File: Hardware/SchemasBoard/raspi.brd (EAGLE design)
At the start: 14.2 x 24.8 mm, 9 parts

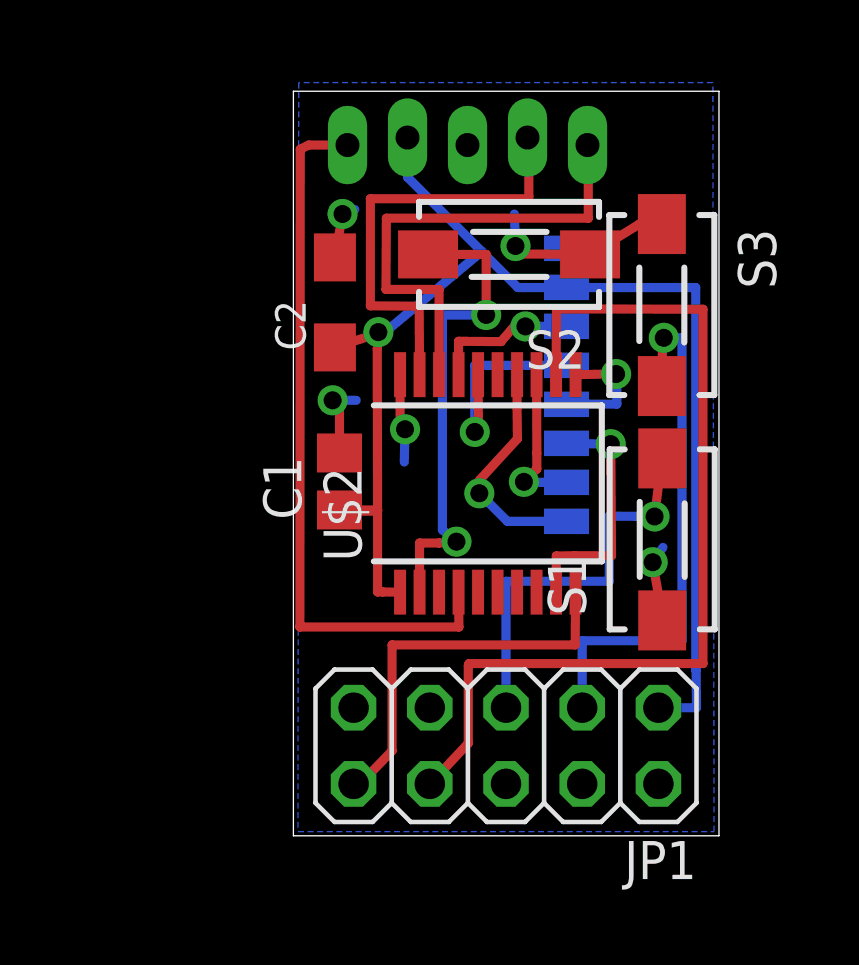
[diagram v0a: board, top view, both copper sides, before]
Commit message: aaa
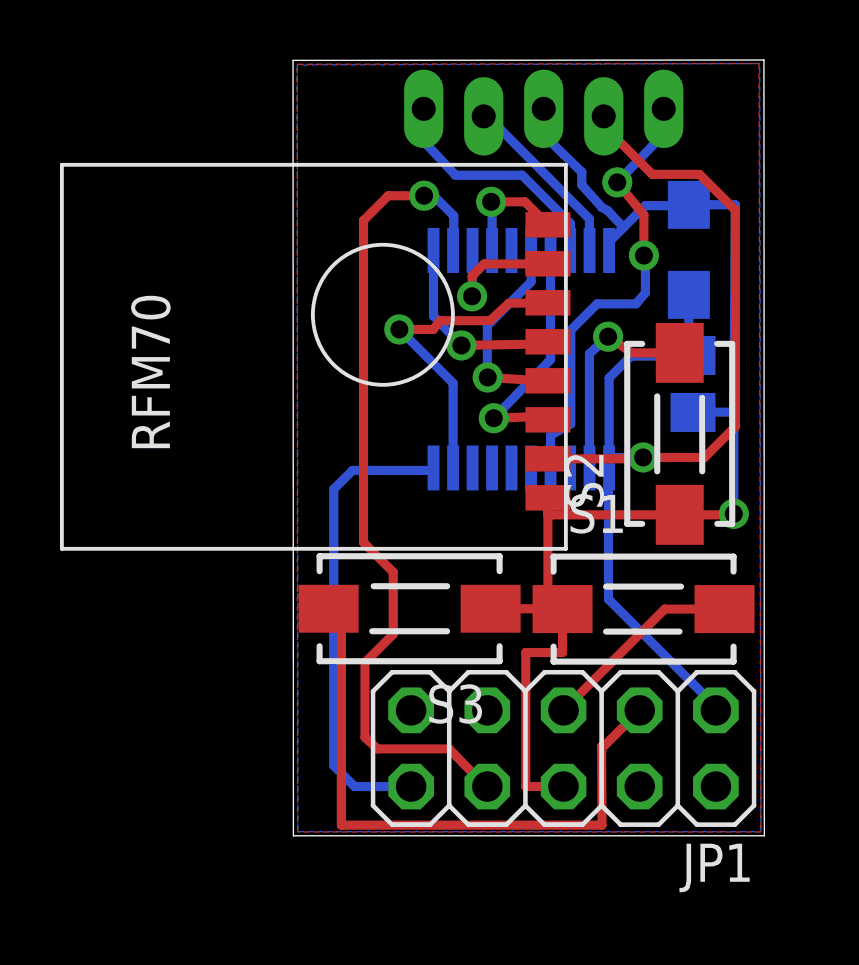
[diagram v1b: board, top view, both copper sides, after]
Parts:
- moved S3 13.2 mm to (3.87, 7.57), turned to 180 degrees
- moved C1 12.2 mm to (13.3, 15.1), flipped to the bottom, turned to 270 degrees
- moved C2 11.9 mm to (13.2, 19.5), flipped to the bottom
- moved S2 8.26 mm to (12.9, 13.4), turned to 90 degrees
- moved U$1 8.14 mm to (-5.82, 11.4), flipped to the top, turned to 90 degrees
- moved U$2 4.29 mm to (7.60, 15.9), flipped to the bottom
- moved U$3 2.81 mm to (8.34, 24.2), turned to 180 degrees
- moved S1 2.41 mm to (11.7, 7.56), turned to 0 degrees
- moved JP1 1.92 mm to (9.00, 2.91)
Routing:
- net GND: track 16.5 -> 43.6 mm, vias 5 -> 1
- net N$28: track 16.4 -> 7.20 mm, vias 2 -> 1
- net N$25: track 24.0 -> 15.1 mm, vias 0 -> 2
- net N$18: track 14.9 -> 6.00 mm
- net N$19: track 16.3 -> 8.03 mm
- net VDD: track 45.7 -> 39.0 mm
- net N$2: track 13.3 -> 6.76 mm, vias 1 -> 0
- net N$21: track 7.74 -> 3.84 mm
- net N$34: track 31.2 -> 27.6 mm, vias 0 -> 1
- net N$16: track 4.96 -> 8.21 mm
- net N$1: track 17.9 -> 20.7 mm, vias 1 -> 0
- net N$33: track 13.1 -> 15.7 mm
- net N$23: track 8.24 -> 10.7 mm
- net N$22: track 4.09 -> 6.45 mm
- added copper zone on layer 1, net VDD
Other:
- board size 14.2 x 24.8 mm -> 15.7 x 25.9 mm
